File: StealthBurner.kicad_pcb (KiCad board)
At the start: 2 copper layers, 44.9 x 31.7 mm, 14 parts, among them J1 PROBE, J2 E-Step, J3 HE, J4 HET, J5 FS, J6 HEF, J7 PCF, J8 LED, J9 MCU, M1 Mount, M2 Mount

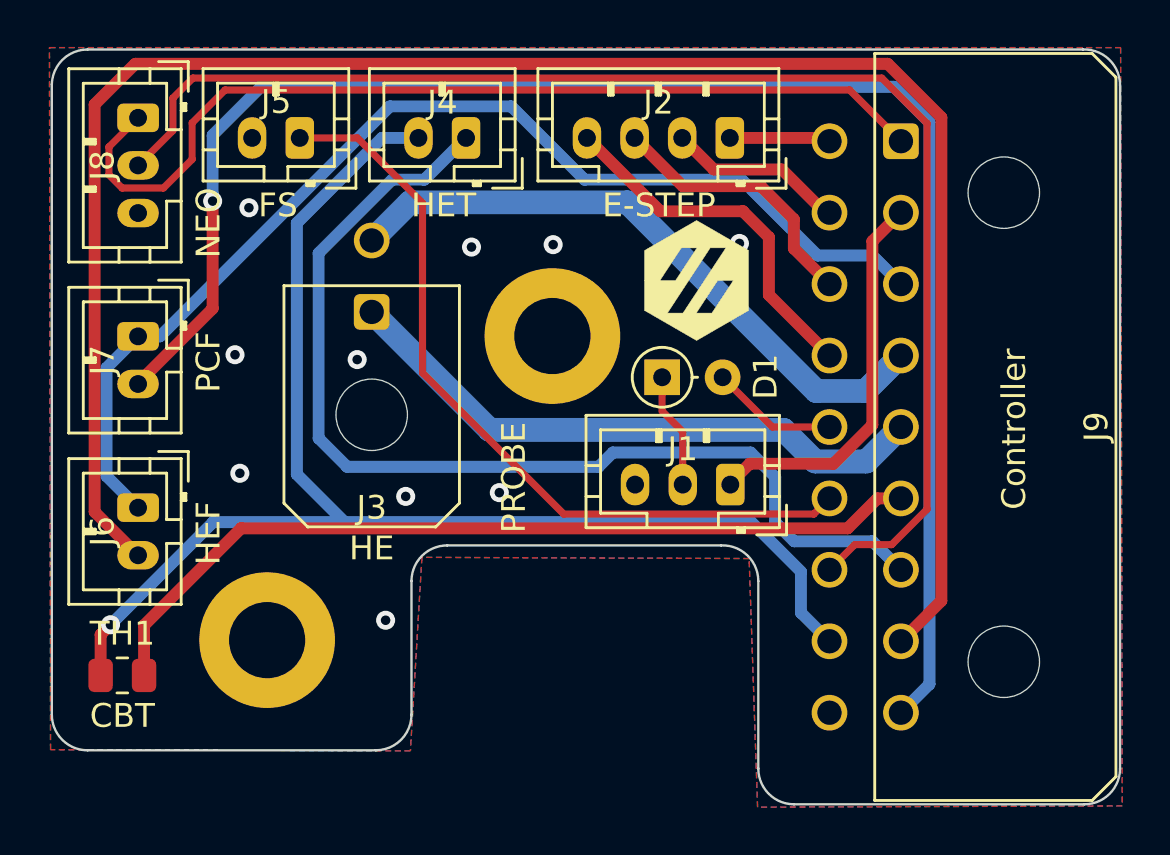
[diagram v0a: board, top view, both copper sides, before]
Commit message: 重新设计 PCB
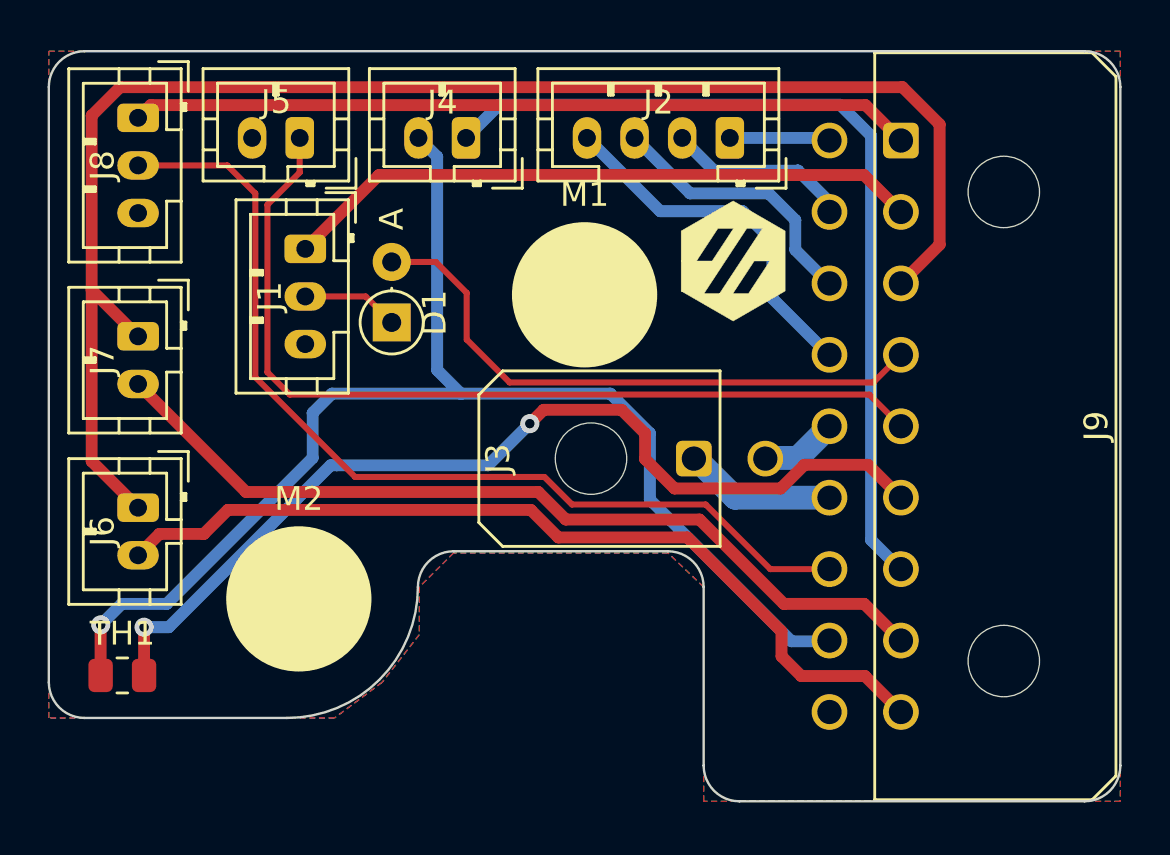
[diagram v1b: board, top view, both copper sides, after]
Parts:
- D1: footprint Diode_THT:D_DO-34_SOD68_P2.54mm_Vertical_AnodeUp -> Diode_THT:D_DO-35_SOD27_P2.54mm_Vertical_AnodeUp
- M1, M2: value Mount -> M3_hole; footprint MountingHole:MountingHole_3.2mm_M3_ISO7380_Pad -> MountingHole:MountingHole_3.2mm_M3_User
- moved J1 20.4 mm to (136.3, 97.3), turned to -90 degrees
- moved M1 19.7 mm to (148.0, 99.2)
- moved M2 15.3 mm to (136.0, 112.0)
- moved J3 14.9 mm to (152.6, 106.1), turned to 90 degrees
- moved D1 11.6 mm to (139.9, 100.4), turned to 90 degrees
- moved G*** 1.74 mm to (154.2, 97.8)
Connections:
- J9 pad 14: /P_SIG -> /HE-
- J9 pad 15: /FS -> /HE+
- J9 pad 4: /HE- -> /P_SIG
- J9 pad 5: /HE+ -> /FS
- J9 pad 8: /HEF -> /PCF
- J9 pad 9: /PCF -> /HEF
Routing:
- net /HEF: track 79.6 -> 37.0 mm
- net /PCF: track 68.6 -> 36.5 mm, vias 1 -> 0
- net /HE-: track 26.8 -> 3.26 mm
- net /P_SIG: track 5.35 -> 25.1 mm
- net /HE+: track 25.4 -> 6.37 mm
- net /DATA: track 57.6 -> 40.6 mm
- net /V_FAN: track 47.4 -> 64.1 mm
- net +24V: track 16.4 -> 26.9 mm
- net /HET: track 44.3 -> 36.9 mm
- net +5V: track 39.9 -> 32.9 mm
- net /FS: track 33.2 -> 37.9 mm
- net /CBT: track 36.1 -> 40.6 mm, vias 0 -> 2
- net GNDA: track 57.3 -> 55.3 mm
- net Net-(D1-Pad1): track 4.87 -> 4.08 mm
- net GND: vias 10 -> 0
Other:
- board size 44.9 x 31.7 mm -> 45 x 31.5 mm
- board text removed: "CBT"
- board text removed: "Controller"
- board text removed: "E-STEP"
- board text removed: "FS"
- board text removed: "HE"
- board text removed: "HEF"
- board text removed: "HET"
- board text removed: "NEO"
- board text removed: "PCF"
- board text removed: "PROBE"

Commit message: 更新到 Beta2
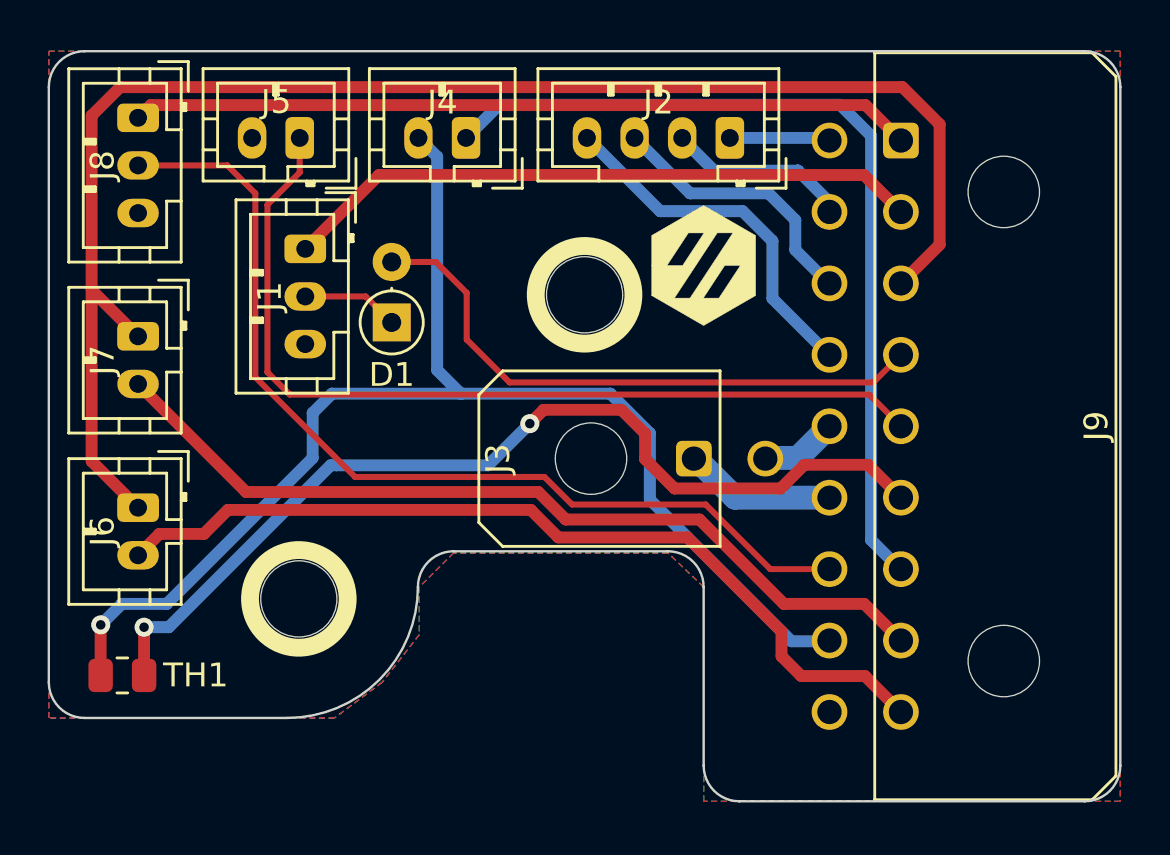
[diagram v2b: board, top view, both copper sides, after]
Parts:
- moved G*** 1.25 mm to (153.0, 98.0)
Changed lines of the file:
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@@
     (title "StealthBurner Toolhead PCB")
     (date "2022-05-24")
-    (rev "Bata0")
+    (rev "Bata1")
     (company "LassiCat Organization")
     (comment 1 "Auther: CharlieYu")
@@
     (property "Sheetname" "")
     (attr smd)
-    (fp_text reference "TH1" (at 0 1.75874) (layer "F.SilkS")
+    (fp_text reference "TH1" (at -3.082812 0.004398) (layer "F.SilkS")
       (effects (font (size 1 1) (thickness 0.15)))
     )
@@
     (property "Sheetname" "")
     (attr through_hole)
-    (fp_text reference "D1" (at 0.41 1.8 90) (layer "F.SilkS")
+    (fp_text reference "D1" (at -2.2 0) (layer "F.SilkS")
       (effects (font (size 1 1) (thickness 0.15)))
     )
@@
       (effects (font (size 1 1) (thickness 0.15)))
     )
-    (fp_text user "A" (at 4.34 0 90) (layer "F.SilkS")
-      (effects (font (size 1 1) (thickness 0.15)))
-    )
-    (fp_text user "A" (at 4.34 0 90) (layer "F.Fab")
-      (effects (font (size 1 1) (thickness 0.15)))
-    )
-    (fp_text user "${REFERENCE}" (at 1.27 -2.326371 90) (layer "F.Fab")
+    (fp_text user "A" (at 4.34 0 90) (layer "F.SilkS") hide
+      (effects (font (size 1 1) (thickness 0.15)))
+    )
+    (fp_text user "A" (at 4.34 0 90) (layer "F.Fab") hide
+      (effects (font (size 1 1) (thickness 0.15)))
+    )
+    (fp_text user "${REFERENCE}" (at 1.27 -2.326371 90) (layer "F.Fab") hide
       (effects (font (size 1 1) (thickness 0.15)))
     )
@@
     (tags "mounting hole 3.2mm no annular m3")
     (attr exclude_from_pos_files exclude_from_bom)
-    (fp_text reference "M2" (at 0 -4.2) (layer "F.SilkS")
-      (effects (font (size 1 1) (thickness 0.15)))
-    )
-    (fp_text value "M3_hole" (at 0 4.2) (layer "F.Fab")
-      (effects (font (size 1 1) (thickness 0.15)))
-    )
-    (fp_text user "${REFERENCE}" (at 0 0) (layer "F.Fab")
-      (effects (font (size 1 1) (thickness 0.15)))
-    )
-    (fp_circle (center 0 0) (end 2.54 0) (layer "Cmts.User") (width 0.15) (fill none))
-    (fp_circle (center 0 0) (end 2.54 0) (layer "F.CrtYd") (width 0.05) (fill none))
+    (fp_text reference "M2" (at 0 -4.2) (layer "F.SilkS") hide
+      (effects (font (size 1 1) (thickness 0.15)))
+    )
+    (fp_text value "M3_hole" (at 0 4.2) (layer "F.Fab") hide
+      (effects (font (size 1 1) (thickness 0.15)))
+    )
+    (fp_text user "${REFERENCE}" (at 0 0) (layer "F.Fab") hide
+      (effects (font (size 1 1) (thickness 0.15)))
+    )
+    (fp_circle (center 0 0) (end 2.05 0) (layer "F.SilkS") (width 0.75) (fill none))
+    (fp_circle (center 0 0) (end 1.6 0) (layer "Cmts.User") (width 0.1) (fill none))
+    (fp_circle (center 0 0) (end 1.6 0) (layer "F.CrtYd") (width 0.1) (fill none))
     (pad "" np_thru_hole circle (at 0 0) (size 3.2 3.2) (drill 3.2) (layers *.Cu *.Mask))
   )
@@
     (tags "mounting hole 3.2mm no annular m3")
     (attr exclude_from_pos_files exclude_from_bom)
-    (fp_text reference "M1" (at 0 -4.2) (layer "F.SilkS")
-      (effects (font (size 1 1) (thickness 0.15)))
-    )
-    (fp_text value "M3_hole" (at 0 4.2) (layer "F.Fab")
-      (effects (font (size 1 1) (thickness 0.15)))
-    )
-    (fp_text user "${REFERENCE}" (at 0 0) (layer "F.Fab")
-      (effects (font (size 1 1) (thickness 0.15)))
-    )
-    (fp_circle (center 0 0) (end 2.54 0) (layer "Cmts.User") (width 0.15) (fill none))
-    (fp_circle (center 0 0) (end 2.54 0) (layer "F.CrtYd") (width 0.05) (fill none))
+    (fp_text reference "M1" (at 0 -4.2) (layer "F.SilkS") hide
+      (effects (font (size 1 1) (thickness 0.15)))
+    )
+    (fp_text value "M3_hole" (at 0 4.2) (layer "F.Fab") hide
+      (effects (font (size 1 1) (thickness 0.15)))
+    )
+    (fp_text user "${REFERENCE}" (at 0 0) (layer "F.Fab") hide
+      (effects (font (size 1 1) (thickness 0.15)))
+    )
+    (fp_circle (center 0 0) (end 2.05 0) (layer "F.SilkS") (width 0.75) (fill none))
+    (fp_circle (center 0 0) (end 1.6 0) (layer "Cmts.User") (width 0.1) (fill none))
+    (fp_circle (center 0 0) (end 1.6 0) (layer "F.CrtYd") (width 0.1) (fill none))
     (pad "" np_thru_hole circle (at 0 0) (size 3.2 3.2) (drill 3.2) (layers *.Cu *.Mask))
   )
@@
   )
   (footprint "Logos:voron_logo_hex" (layer "F.Cu")
-    (at 154.24 97.81)
+    (at 153 98)
     (attr board_only exclude_from_pos_files exclude_from_bom)
     (fp_text reference "G***" (at 0 0) (layer "F.SilkS") hide
@@
     )
   )
-  (gr_circle (center 148 99.23) (end 151 99.23) (layer "F.SilkS") (width 0.1) (fill solid))
-  (gr_circle (center 136 112) (end 139 112) (layer "F.SilkS") (width 0.1) (fill solid))
   (gr_line (start 125.5 90.5) (end 125.5 115.5) (layer "Edge.Cuts") (width 0.1))
   (gr_line (start 170.5 119) (end 170.5 90.5) (layer "Edge.Cuts") (width 0.1))
@@
   (group "" (id 138ee650-507a-4b6c-aa52-9a524f6554fc)
     (members
-      3c19eee8-8ef9-4c6e-b5af-9f26817e96ee
-      88c53001-83db-453f-916c-506f3ad8d7eb
       d2e33ac6-8ba1-45b4-a4e6-6e1f013e565c
       d51818f7-3221-478a-8396-f76ef6cf744f
